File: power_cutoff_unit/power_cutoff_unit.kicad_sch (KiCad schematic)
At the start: 25 parts, among them J1 Conn_01x02, J2 Conn_01x02, K2 T9GS1L14-5, Q1 AO3400A, SW1 SW_DIP_x02, U1 MOUDLE-SEEEDUINO-XIAO-ESP32C3, U2 STM32G431K8Tx, U3 ADuM1250, U4 ADuM120N, U6 LMZ14201H

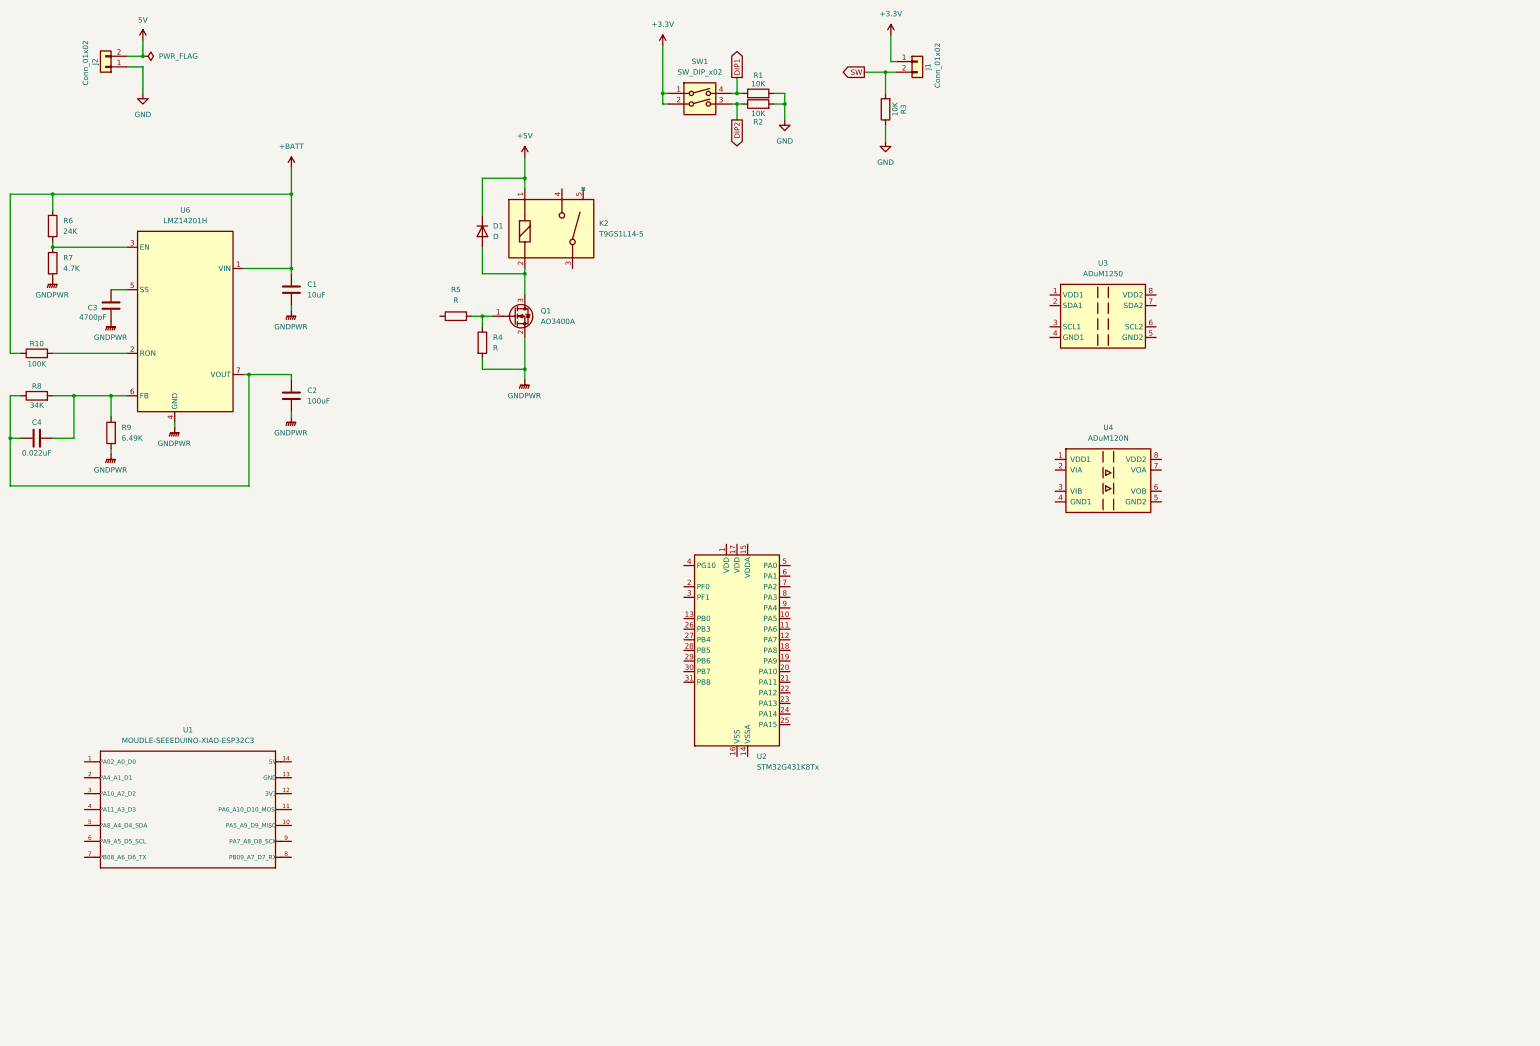
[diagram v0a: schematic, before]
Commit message: 難しくてわかんないッピ
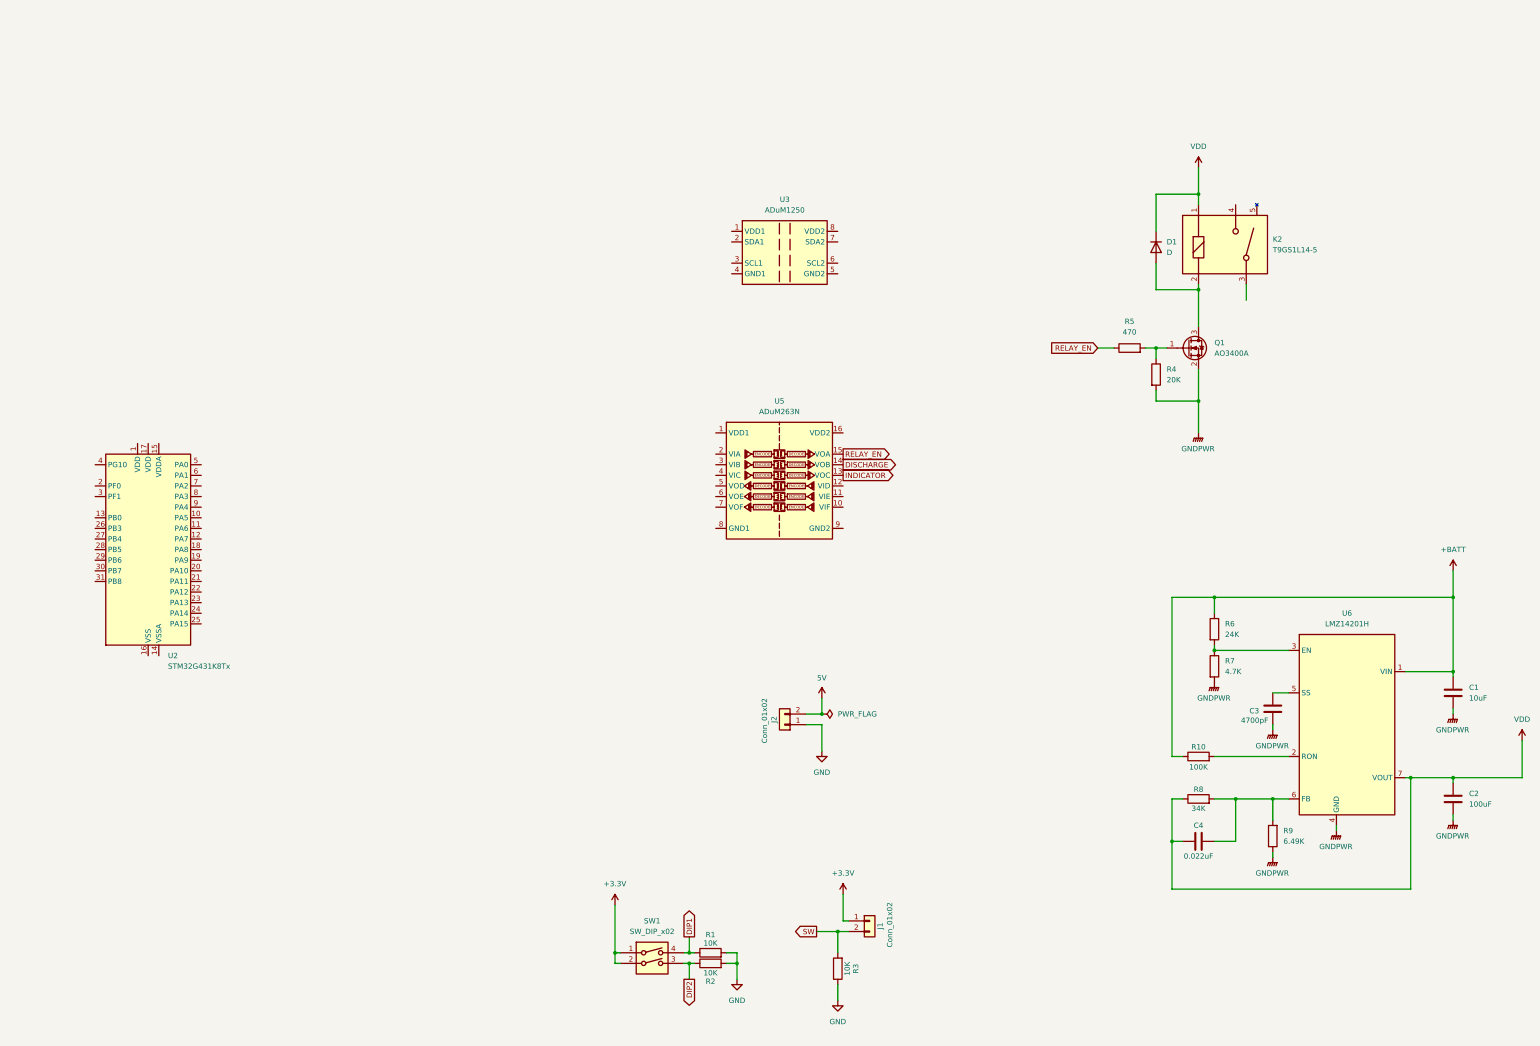
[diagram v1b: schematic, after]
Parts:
- removed U1: MOUDLE-SEEEDUINO-XIAO-ESP32C3, MOUDLE14P-SMD-2.54-21X17.8MM, symbol MOUDLE-SEEEDUINO-XIAO-ESP32C3:MOUDLE-SEEEDUINO-XIAO-ESP32C3
- removed U4: ADuM120N, Package_SO:SOIC-8_3.9x4.9mm_P1.27mm, symbol Isolator:ADuM120N
- added U5: ADuM263N, Package_SO:SOIC-16W_7.5x12.8mm_P1.27mm, symbol Isolator:ADuM263N
- R4: value R -> 20K
- R5: value R -> 470
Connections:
- net +5V is gone; now on net VDD: D1.1 (K), K2.1
- net VDD: now reaches C2.1, C4.1, R8.1, U6.7 (VOUT)
- net RELAY_EN: now reaches R5.1
- net RELAY_EN: now also U5.15 (VOA)
- new net DISCHARGE: U5.14 (VOB)
- new net INDICATOR: U5.13 (VOC)
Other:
- moved on the sheet: C1, C2, C3, C4, D1, J1, J2, K2, Q1, R1, R10, R2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

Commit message: 尽きた
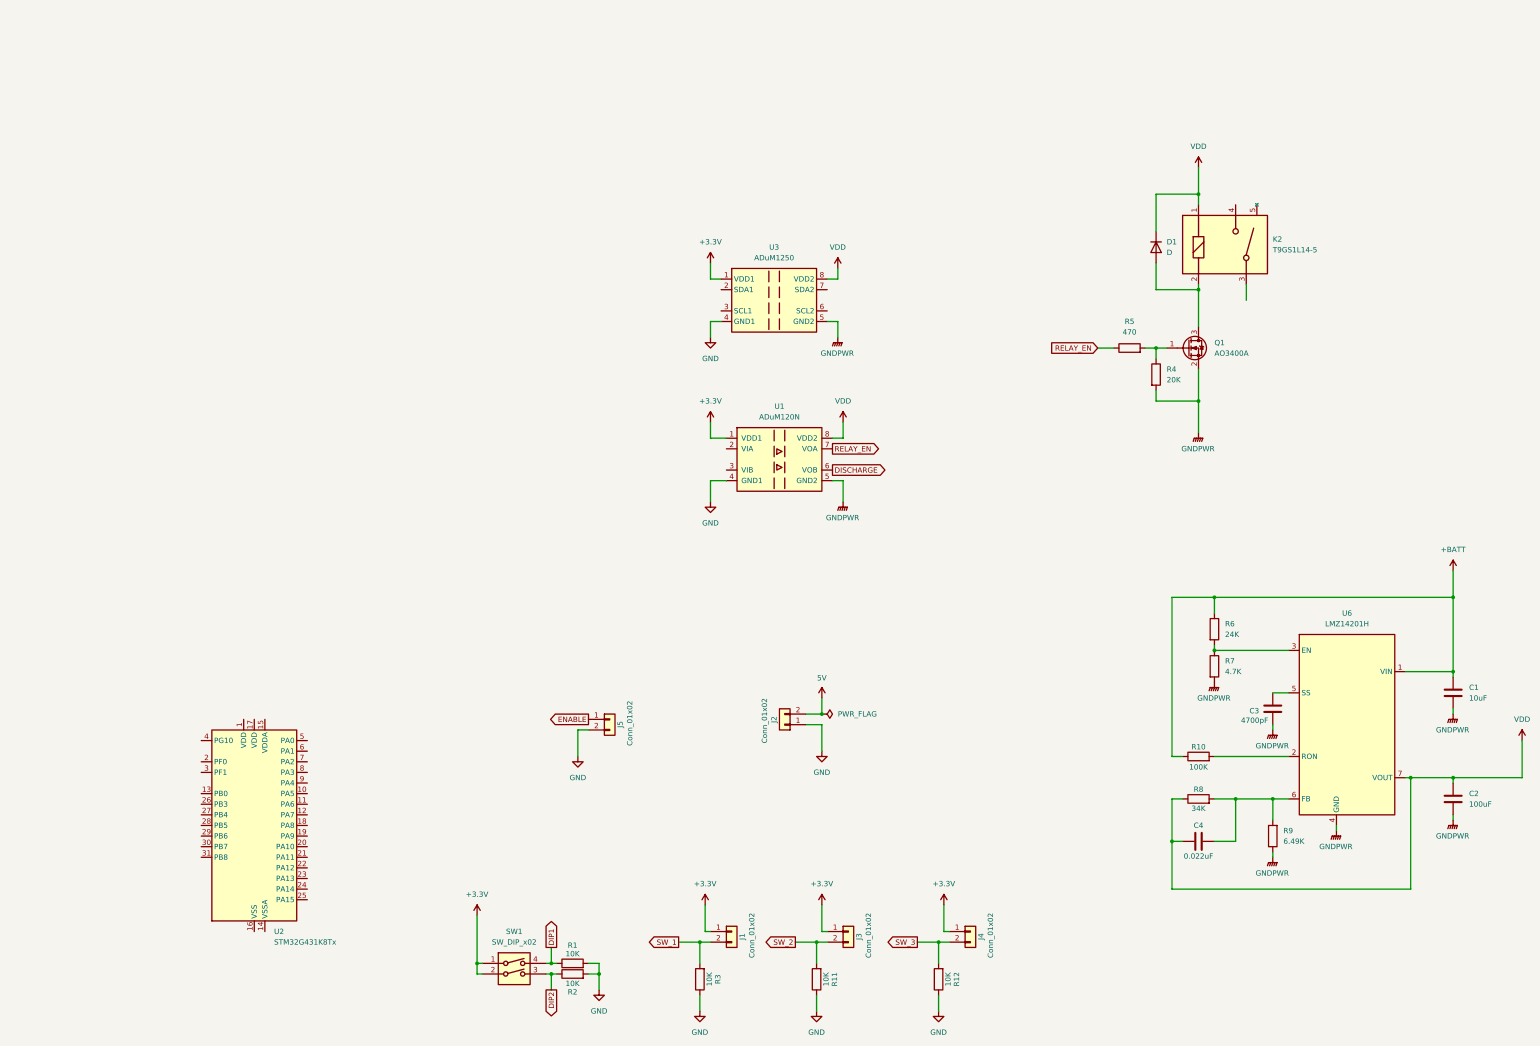
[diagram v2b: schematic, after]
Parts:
- removed U5: ADuM263N, Package_SO:SOIC-16W_7.5x12.8mm_P1.27mm, symbol Isolator:ADuM263N
- added J3, J4, J5: Conn_01x02, Connector_JST:JST_XH_S2B-XH-A_1x02_P2.50mm_Horizontal, symbol Connector_Generic:Conn_01x02
- added R11, R12: 10K, Resistor_SMD:R_0603_1608Metric, symbol Device:R
- added U1: ADuM120N, Package_SO:SOIC-8_3.9x4.9mm_P1.27mm, symbol Isolator:ADuM120N
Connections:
- net +3.3V: now also U3.1 (VDD1), J3.1 (Pin_1), J4.1 (Pin_1), U1.1 (VDD1)
- net DISCHARGE: now also U1.6 (VOB)
- net GND: now also U3.4 (GND1), J5.2 (Pin_2), R11.1, R12.1, U1.4 (GND1)
- net GNDPWR: now also U3.5 (GND2), U1.5 (GND2)
- net RELAY_EN: now also U1.7 (VOA)
- net VDD: now also U3.8 (VDD2), U1.8 (VDD2)
- net SW renamed SW_1
- new net ENABLE: J5.1 (Pin_1)
- new net SW_2: J3.2 (Pin_2), R11.2
- new net SW_3: J4.2 (Pin_2), R12.2
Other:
- moved on the sheet: J1, R1, R2, R3, SW1, U2, U3
